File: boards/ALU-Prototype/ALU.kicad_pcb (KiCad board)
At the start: 2 copper layers, 69.2 x 57.2 mm, 60 parts

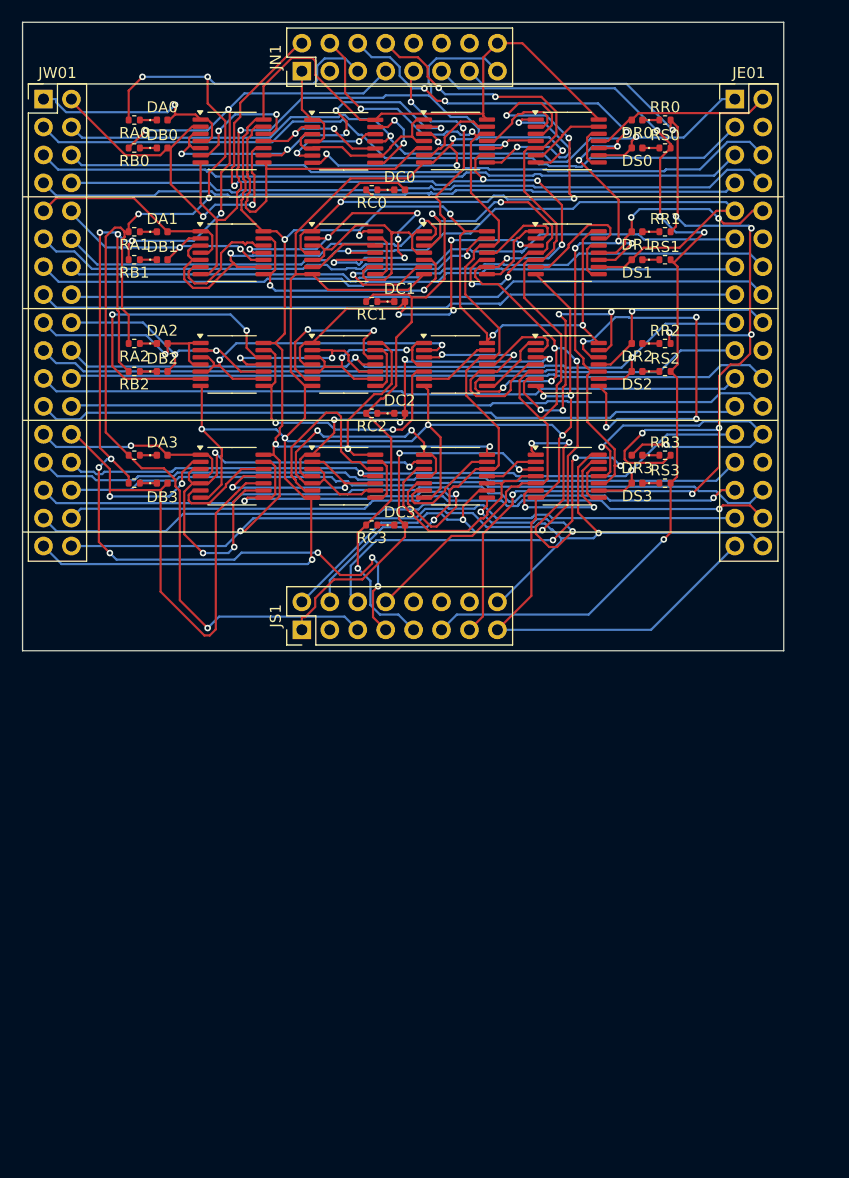
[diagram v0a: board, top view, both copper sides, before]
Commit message: 8-bit PCB, P1 version
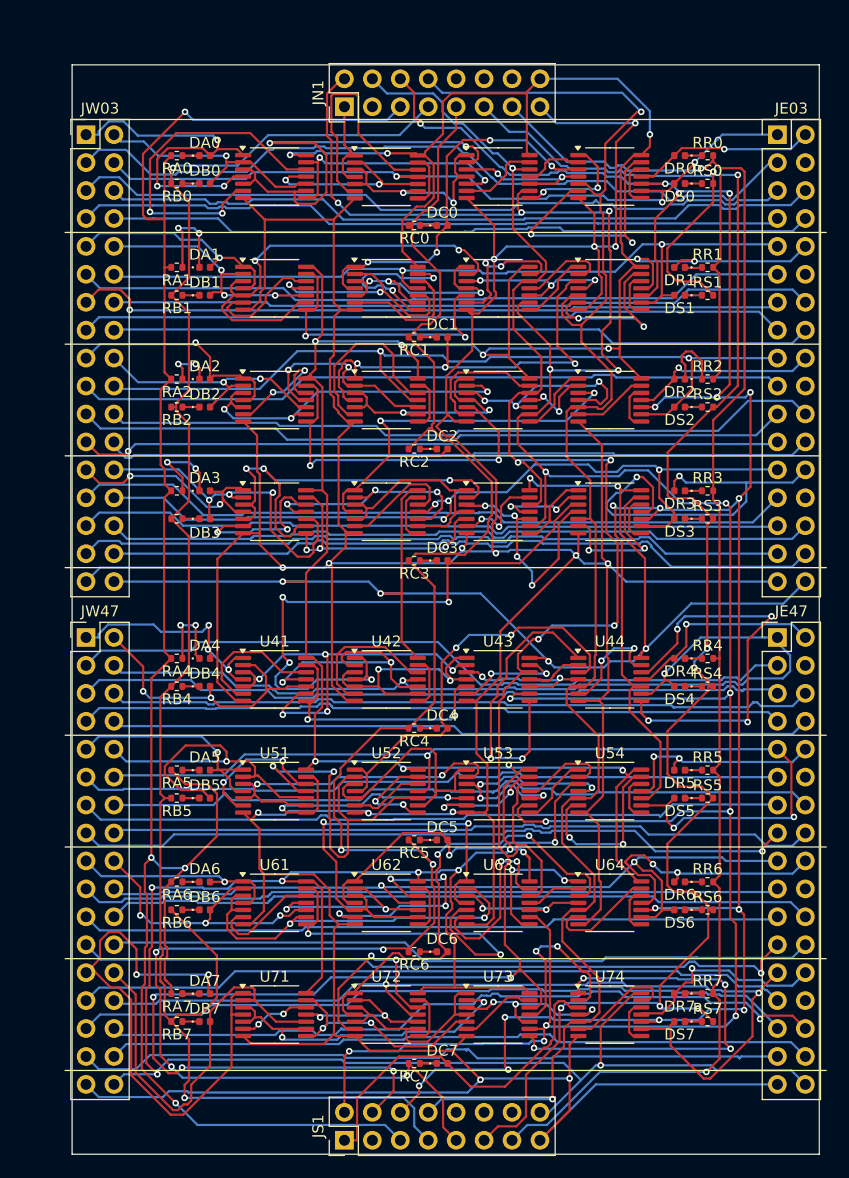
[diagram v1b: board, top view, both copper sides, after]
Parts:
- added DA4: ~, LED_SMD:LED_0402_1005Metric, F.Cu at (29.8, 71.8)
- added DA5: ~, LED_SMD:LED_0402_1005Metric, F.Cu at (29.8, 81.9)
- added DA6: ~, LED_SMD:LED_0402_1005Metric, F.Cu at (29.8, 92.1)
- added DA7: ~, LED_SMD:LED_0402_1005Metric, F.Cu at (29.8, 102.2)
- added DB4: ~, LED_SMD:LED_0402_1005Metric, F.Cu at (29.8, 74.3)
- added DB5: ~, LED_SMD:LED_0402_1005Metric, F.Cu at (29.8, 84.5)
- added DB6: ~, LED_SMD:LED_0402_1005Metric, F.Cu at (29.8, 94.6)
- added DB7: ~, LED_SMD:LED_0402_1005Metric, F.Cu at (29.8, 104.8)
- added DC4: ~, LED_SMD:LED_0402_1005Metric, F.Cu at (51.4, 78.1)
- added DC5: ~, LED_SMD:LED_0402_1005Metric, F.Cu at (51.4, 88.3)
- added DC6: ~, LED_SMD:LED_0402_1005Metric, F.Cu at (51.4, 98.4)
- added DC7: ~, LED_SMD:LED_0402_1005Metric, F.Cu at (51.4, 108.6)
- added DR4: ~, LED_SMD:LED_0402_1005Metric, F.Cu at (73.0, 71.8)
- added DR5: ~, LED_SMD:LED_0402_1005Metric, F.Cu at (73.0, 81.9)
- added DR6: ~, LED_SMD:LED_0402_1005Metric, F.Cu at (73.0, 92.1)
- added DR7: ~, LED_SMD:LED_0402_1005Metric, F.Cu at (73.0, 102.2)
- added DS4: ~, LED_SMD:LED_0402_1005Metric, F.Cu at (73.0, 74.3)
- added DS5: ~, LED_SMD:LED_0402_1005Metric, F.Cu at (73.0, 84.5)
- added DS6: ~, LED_SMD:LED_0402_1005Metric, F.Cu at (73.0, 94.6)
- added DS7: ~, LED_SMD:LED_0402_1005Metric, F.Cu at (73.0, 104.8)
- added JE47: ~, Connector_PinHeader_2.54mm:PinHeader_2x17_P2.54mm_Vertical, F.Cu at (81.9, 69.9)
- added JW47: ~, Connector_PinHeader_2.54mm:PinHeader_2x17_P2.54mm_Vertical, F.Cu at (19.1, 69.9)
- added RA4: 330, Resistor_SMD:R_0402_1005Metric, F.Cu at (27.3, 71.8)
- added RA5: 330, Resistor_SMD:R_0402_1005Metric, F.Cu at (27.3, 81.9)
- added RA6: 330, Resistor_SMD:R_0402_1005Metric, F.Cu at (27.3, 92.1)
- added RA7: 330, Resistor_SMD:R_0402_1005Metric, F.Cu at (27.3, 102.2)
- added RB4: 330, Resistor_SMD:R_0402_1005Metric, F.Cu at (27.3, 74.3)
- added RB5: 330, Resistor_SMD:R_0402_1005Metric, F.Cu at (27.3, 84.5)
- added RB6: 330, Resistor_SMD:R_0402_1005Metric, F.Cu at (27.3, 94.6)
- added RB7: 330, Resistor_SMD:R_0402_1005Metric, F.Cu at (27.3, 104.8)
- added RC4: 330, Resistor_SMD:R_0402_1005Metric, F.Cu at (48.9, 78.1)
- added RC5: 330, Resistor_SMD:R_0402_1005Metric, F.Cu at (48.9, 88.3)
- added RC6: 330, Resistor_SMD:R_0402_1005Metric, F.Cu at (48.9, 98.4)
- added RC7: 330, Resistor_SMD:R_0402_1005Metric, F.Cu at (48.9, 108.6)
- added RR4: 330, Resistor_SMD:R_0402_1005Metric, F.Cu at (75.6, 71.8)
- added RR5: 330, Resistor_SMD:R_0402_1005Metric, F.Cu at (75.6, 81.9)
- added RR6: 330, Resistor_SMD:R_0402_1005Metric, F.Cu at (75.6, 92.1)
- added RR7: 330, Resistor_SMD:R_0402_1005Metric, F.Cu at (75.6, 102.2)
- added RS4: 330, Resistor_SMD:R_0402_1005Metric, F.Cu at (75.6, 74.3)
- added RS5: 330, Resistor_SMD:R_0402_1005Metric, F.Cu at (75.6, 84.5)
- added RS6: 330, Resistor_SMD:R_0402_1005Metric, F.Cu at (75.6, 94.6)
- added RS7: 330, Resistor_SMD:R_0402_1005Metric, F.Cu at (75.6, 104.8)
- added U41: ~, Package_SO:TSSOP-14_4.4x5mm_P0.65mm, F.Cu at (36.2, 73.7)
- added U42: ~, Package_SO:TSSOP-14_4.4x5mm_P0.65mm, F.Cu at (46.4, 73.7)
- added U43: ~, Package_SO:TSSOP-14_4.4x5mm_P0.65mm, F.Cu at (56.5, 73.7)
- added U44: ~, Package_SO:TSSOP-14_4.4x5mm_P0.65mm, F.Cu at (66.7, 73.7)
- added U51: ~, Package_SO:TSSOP-14_4.4x5mm_P0.65mm, F.Cu at (36.2, 83.8)
- added U52: ~, Package_SO:TSSOP-14_4.4x5mm_P0.65mm, F.Cu at (46.4, 83.8)
- added U53: ~, Package_SO:TSSOP-14_4.4x5mm_P0.65mm, F.Cu at (56.5, 83.8)
- added U54: ~, Package_SO:TSSOP-14_4.4x5mm_P0.65mm, F.Cu at (66.7, 83.8)
- added U61: ~, Package_SO:TSSOP-14_4.4x5mm_P0.65mm, F.Cu at (36.2, 94.0)
- added U62: ~, Package_SO:TSSOP-14_4.4x5mm_P0.65mm, F.Cu at (46.4, 94.0)
- added U63: ~, Package_SO:TSSOP-14_4.4x5mm_P0.65mm, F.Cu at (56.5, 94.0)
- added U64: ~, Package_SO:TSSOP-14_4.4x5mm_P0.65mm, F.Cu at (66.7, 94.0)
- added U71: ~, Package_SO:TSSOP-14_4.4x5mm_P0.65mm, F.Cu at (36.2, 104.1)
- added U72: ~, Package_SO:TSSOP-14_4.4x5mm_P0.65mm, F.Cu at (46.4, 104.1)
- added U73: ~, Package_SO:TSSOP-14_4.4x5mm_P0.65mm, F.Cu at (56.5, 104.1)
- added U74: ~, Package_SO:TSSOP-14_4.4x5mm_P0.65mm, F.Cu at (66.7, 104.1)
- moved JS1 46.6 mm to (42.5, 115.6)
- moved RR2 5.04 mm to (75.6, 46.4)
- moved RS1 5.04 mm to (75.6, 38.7)
- moved RS3 5.04 mm to (75.6, 59.1)
- moved RR0 5.04 mm to (75.6, 26.0)
- moved RS0 5.04 mm to (75.6, 28.6)
- moved RR1 5.04 mm to (75.6, 36.2)
- moved RR3 5.04 mm to (75.6, 56.5)
- moved RS2 5.04 mm to (75.6, 48.9)
- moved DC0 5.04 mm to (51.4, 32.4)
- moved DC2 5.04 mm to (51.4, 52.7)
- moved RA2 5.04 mm to (27.3, 46.4)
- moved RB1 5.04 mm to (27.3, 38.7)
- moved RB3 5.04 mm to (27.3, 59.1)
- moved RC0 5.04 mm to (48.9, 32.4)
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- renumbered JE01 to JE03, JW01 to JW03
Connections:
- DC3 pad 2: C -> /ALUSlice3/C
- U34 pad 3: C -> /ALUSlice3/C
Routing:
- net VDD: track 269.6 -> 536.9 mm, vias 10 -> 25
- net GND: track 299.1 -> 518.3 mm, vias 12 -> 15
- net SUB: track 80.4 -> 213.2 mm, vias 3 -> 9
- net ADD: track 135.5 -> 253.3 mm, vias 11 -> 15
- net XOR: track 114.8 -> 230.5 mm, vias 11 -> 17
- net GNDC: track 75.9 -> 179.1 mm, vias 3 -> 6
- net S5: track 0.00 -> 89.3 mm, vias 0 -> 3
- net S7: track 0.00 -> 86.3 mm, vias 0 -> 2
- net S4: track 0.00 -> 85.5 mm, vias 0 -> 2
- net GNDS: track 89.4 -> 166.7 mm, vias 4 -> 7
- net S6: track 0.00 -> 75.5 mm, vias 0 -> 2
- net PD7: track 0.00 -> 67.6 mm, vias 0 -> 1
- net PB7: track 0.00 -> 66.5 mm
- net PA4: track 0.00 -> 66.4 mm
- net PD5: track 0.00 -> 66.3 mm
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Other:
- board size 69.2 x 57.2 mm -> 67.9 x 99.1 mm
